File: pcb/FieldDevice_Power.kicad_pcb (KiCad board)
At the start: 2 copper layers, 22.9 x 20.6 mm, 14 parts, among them J1 Vin, J2 Vout, U1 LM2621

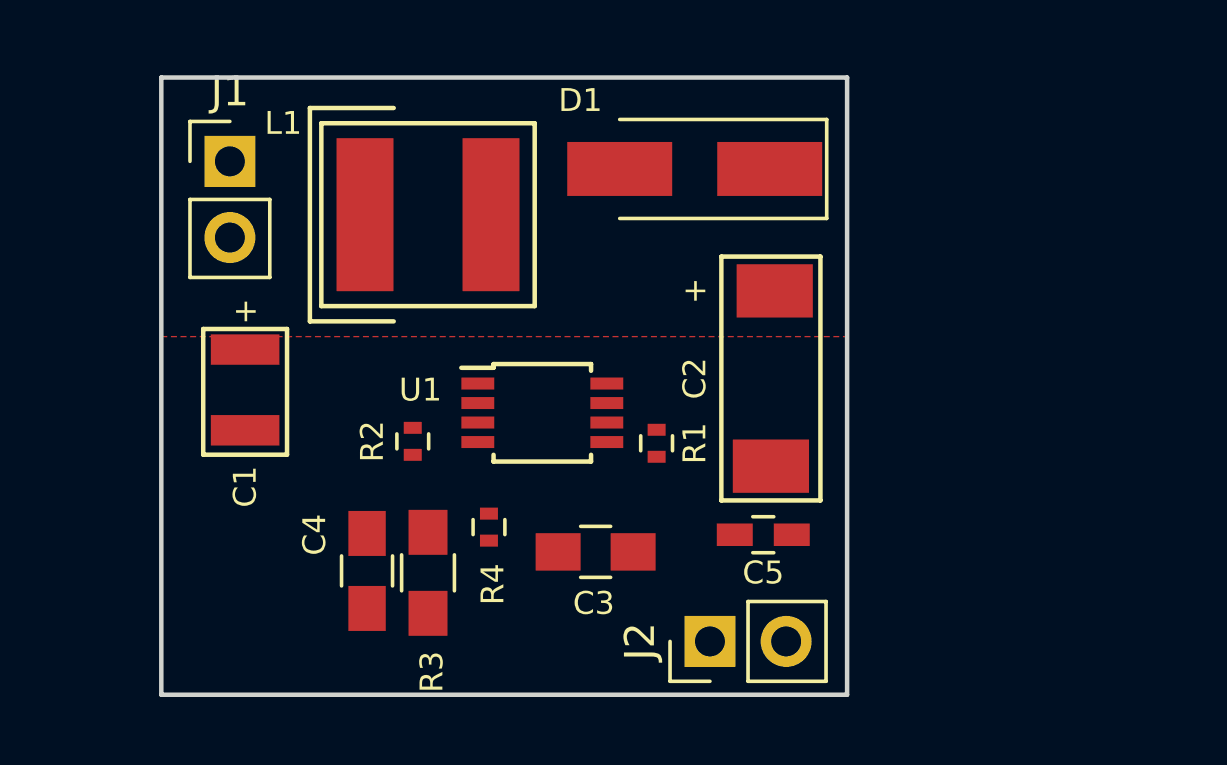
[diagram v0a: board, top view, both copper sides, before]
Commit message: Completed the layout and parts decisions
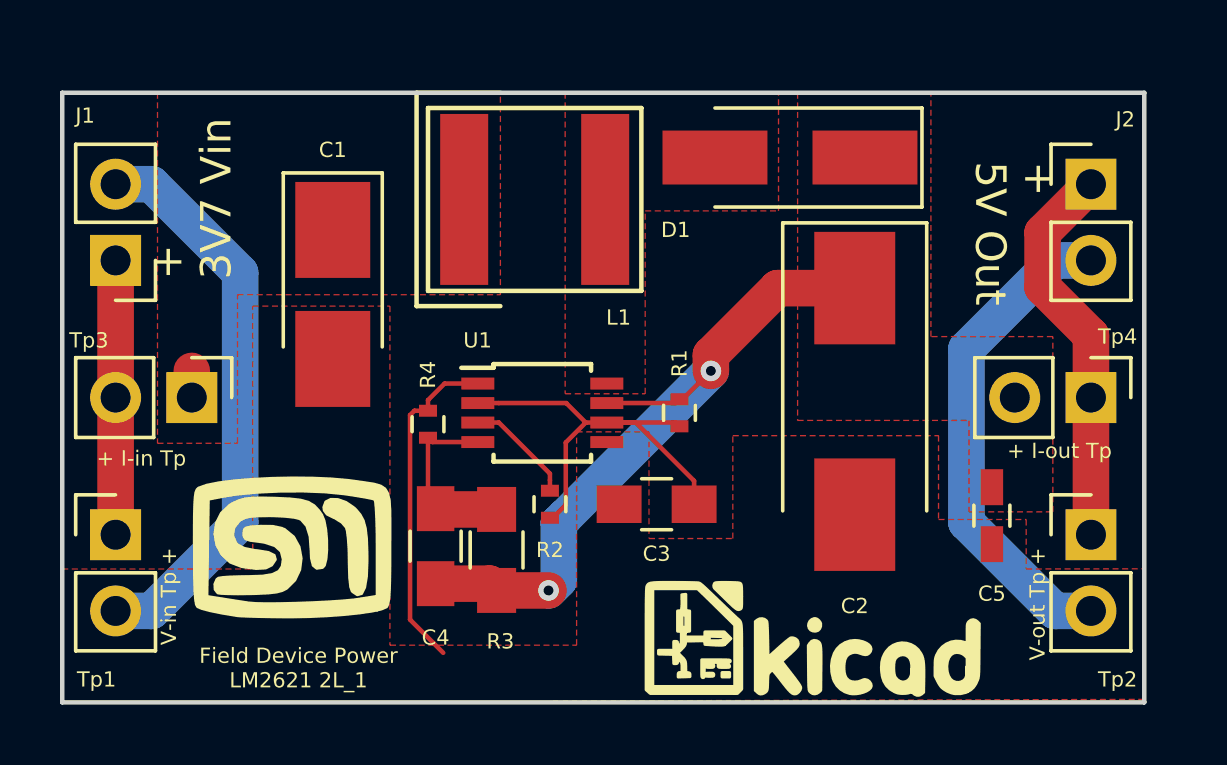
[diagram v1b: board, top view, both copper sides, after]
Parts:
- added G***: LOGO, FieldDevice_Power:MyBasic_rounded_50_1, B.Cu at (180.8, 100.5)
- added G***: LOGO, FieldDevice_Power:MyBasic_rounded_50_1, F.Cu at (170.2, 111.6)
- added G***: LOGO, FieldDevice_Power:KiCad-Logo, F.Cu at (187.6, 114.7)
- added REF***: KiCad-Logo2_6mm_SilkScreen, Symbols:KiCad-Logo2_6mm_SilkScreen, B.Cu at (180.8, 113.4)
- added Tp1: VinTest, Pin_Headers:Pin_Header_Straight_1x02_Pitch2.54mm, F.Cu at (164.3, 111.3)
- added Tp2: VoutTest, Pin_Headers:Pin_Header_Straight_1x02_Pitch2.54mm, F.Cu at (196.8, 111.3)
- added Tp3: IinTest, Pin_Headers:Pin_Header_Straight_1x02_Pitch2.54mm, F.Cu at (166.9, 106.7)
- added Tp4: IoutTest, Pin_Headers:Pin_Header_Straight_1x02_Pitch2.54mm, F.Cu at (196.8, 106.7)
- C1: footprint FieldDevice_Power:Capacitor_1411 -> Capacitors_Tantalum_SMD:CP_Tantalum_Case-B_EIA-3528-21_Hand
- C2: value 68μF -> 100μF; footprint FieldDevice_Power:Capacitor_2917 -> Capacitors_Tantalum_SMD:CP_Tantalum_Case-D_EIA-7343-31_Hand
- C3: value 100nF 16V -> 1uF 16V
- L1: footprint FieldDevice_Power:INDUCTOR_VLS6045EX-6R8M -> FieldDevice_Power:INDUCTOR_1255AY-6R8M=P3
- R1: value 500Ω -> 48.7Ω
- R2: value 200kΩ -> 357kΩ E96, 1%
- R4: value 50kΩ -> 49.9kΩ E96 1%
- moved J2 19.8 mm to (196.8, 99.6), turned to 0 degrees
- moved C5 7.65 mm to (193.5, 110.6), turned to 90 degrees
- moved J1 5.04 mm to (164.3, 102.1), turned to 180 degrees
- moved R2 5.03 mm to (178.8, 110.2), turned to 270 degrees
- moved C1 4.32 mm to (171.6, 103.2)
- moved R4 3.99 mm to (174.8, 107.6), turned to 270 degrees
- moved L1 3.59 mm to (178.3, 100.1)
- moved D1 3.20 mm to (186.8, 98.7)
- moved C2 2.77 mm to (189.0, 106.8)
- moved C3 2.58 mm to (182.4, 110.2)
- moved C4 2.43 mm to (175.0, 111.6)
- moved R3 2.41 mm to (177.0, 111.8)
- moved R1 1.27 mm to (183.1, 107.2)
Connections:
- C1 pad 1: /Vin -> /Vin1
- C2 pad 1: /Vout -> /Vout1
- C4 pad 1: /Vout -> /Vout1
- C5 pad 2: /Vout -> /Vout1
- D1 pad 1: /Vout -> /Vout1
- L1 pad 1: /Vin -> /Vin1
- R1 pad 2: /Vout -> /Vout1
- R3 pad 1: /Vout -> /Vout1
- U1 pad 7: /Vout -> /Vout1
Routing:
- net GND: track 0.00 -> 46.9 mm
- net /Vout1: track 0.00 -> 23.6 mm, vias 0 -> 2
- net Net-(C3-Pad2): track 0.00 -> 15.3 mm
- net /Vout: track 0.00 -> 13.0 mm
- net /Vin: track 0.00 -> 8.38 mm
- net Net-(C4-Pad2): track 0.00 -> 6.23 mm
- net Net-(R2-Pad1): track 0.00 -> 3.68 mm
- net /Vin1: track 0.00 -> 0.89 mm
- added copper zone on F.Cu, net /Vin1
- added copper zone on F.Cu, net /Vout1
- added copper zone on F.Cu, net Net-(D1-Pad2)
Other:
- board size 22.9 x 20.6 mm -> 36.1 x 20.3 mm
- net class Default: clearance 0.2 -> 0.1524; trace_width 0.25 -> 0.1524; via_dia 0.6 -> 0.6858; via_drill 0.4 -> 0.3302
- rule pad_to_mask_clearance: 0.2 -> 0
- rule trace_clearance: 0.2 -> 0.1524
- rule trace_min: 0.2 -> 0.1524
- rule via_min_drill: 0.3 -> 0.3302
- rule via_min_size: 0.4 -> 0.6858
- board text added: "+ 3V7 Vin"
- board text added: "+ 5V Out"
- board text added: "+ I-in Tp"
- board text added: "+ I-out Tp"
- board text added: "Field Device Power LM2621 2L_1"
- board text added: "V-in Tp +"
- board text added: "V-out Tp +"
